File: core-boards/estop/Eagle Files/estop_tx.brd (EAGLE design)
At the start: 76.2 x 50.8 mm, 32 parts, among them J1 RFM95W-3072, J2 JST-XH-02-PIN-ROUND-PAD, J3 JST-XH-02-PIN-ROUND-PAD, J4 JST-XH-02-PIN-ROUND-PAD, J5 JST-XH-02-PIN-ROUND-PAD, J6 B2PS-VH(LF)(SN), U1 R-78E5.0-1.0CONV_R-78E5.0-1.0, U2 TXB0106PWR, U4 ATMEGA328P-AUR

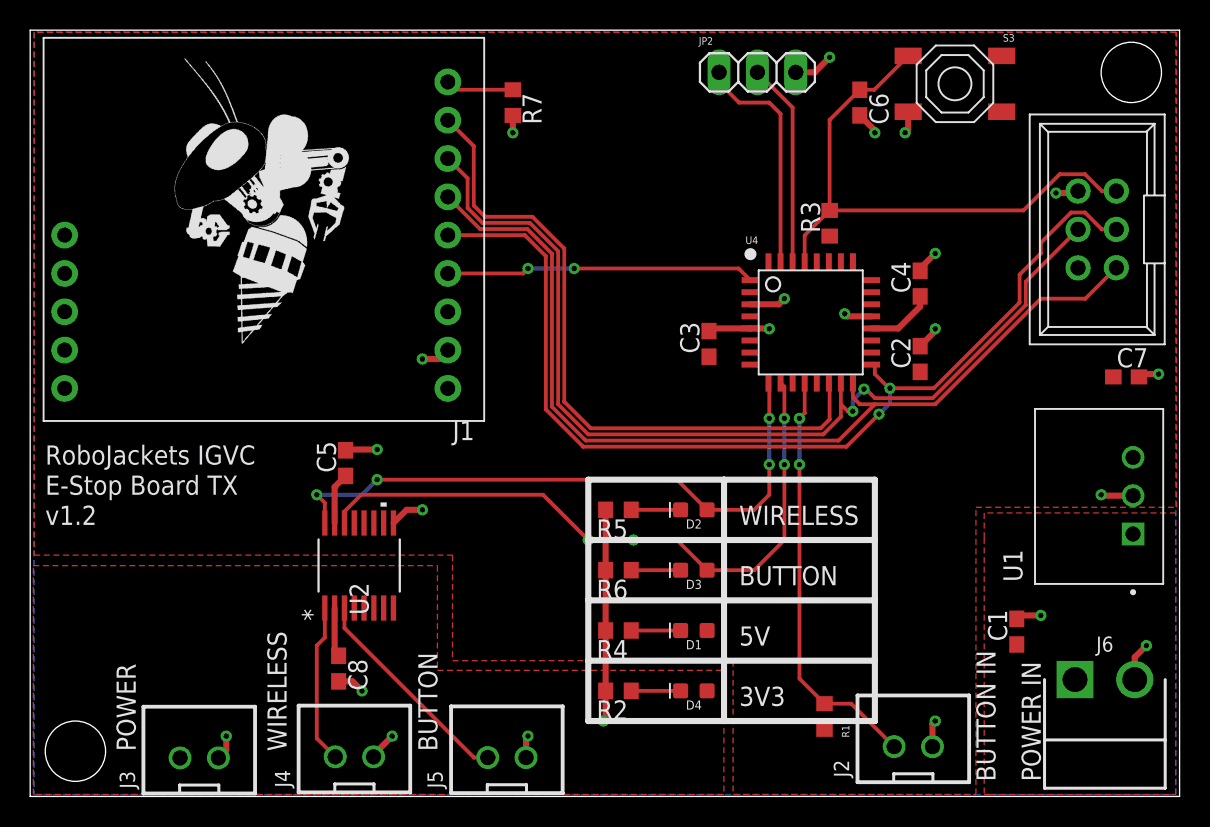
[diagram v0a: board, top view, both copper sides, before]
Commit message: final tm edits for design review
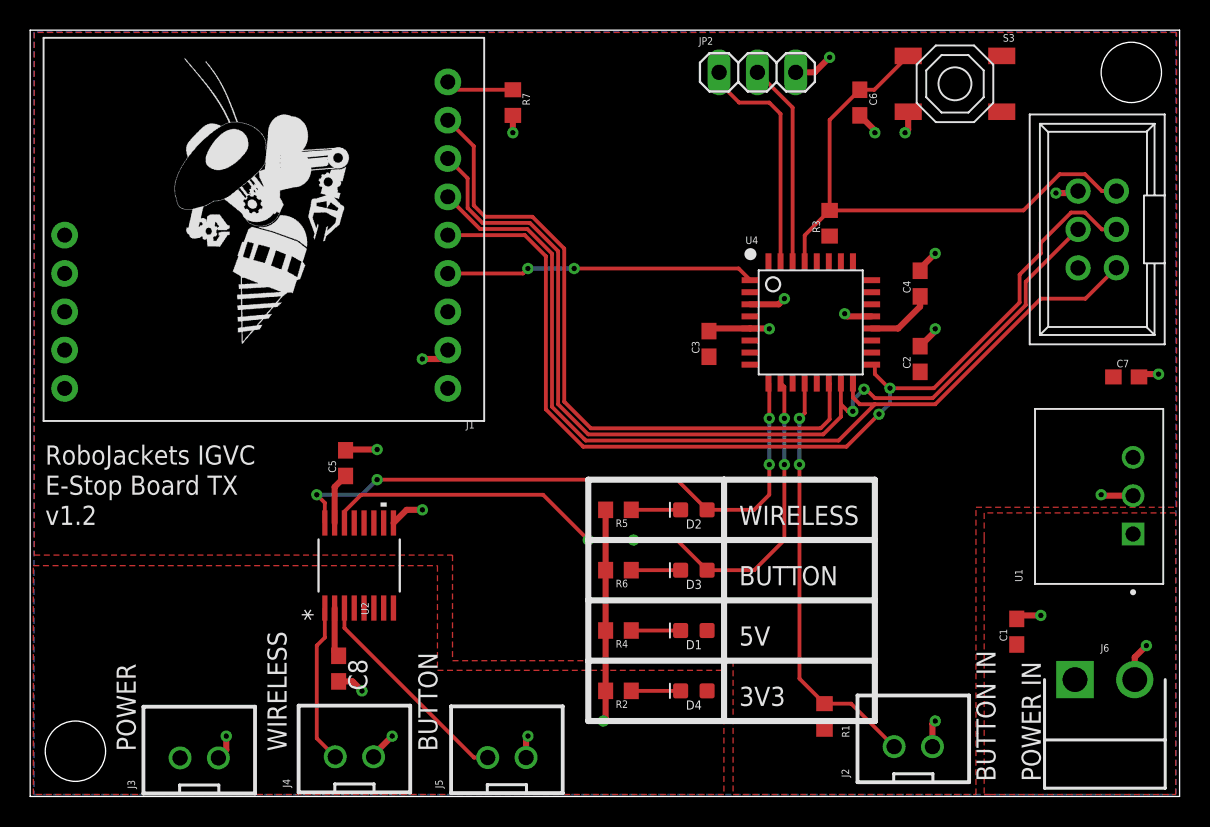
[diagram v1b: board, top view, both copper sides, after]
